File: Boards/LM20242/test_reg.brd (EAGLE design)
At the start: 160 x 100 mm, 12 parts, among them U1 TI_NATIONAL_SEMICONDUCTOR_LM2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

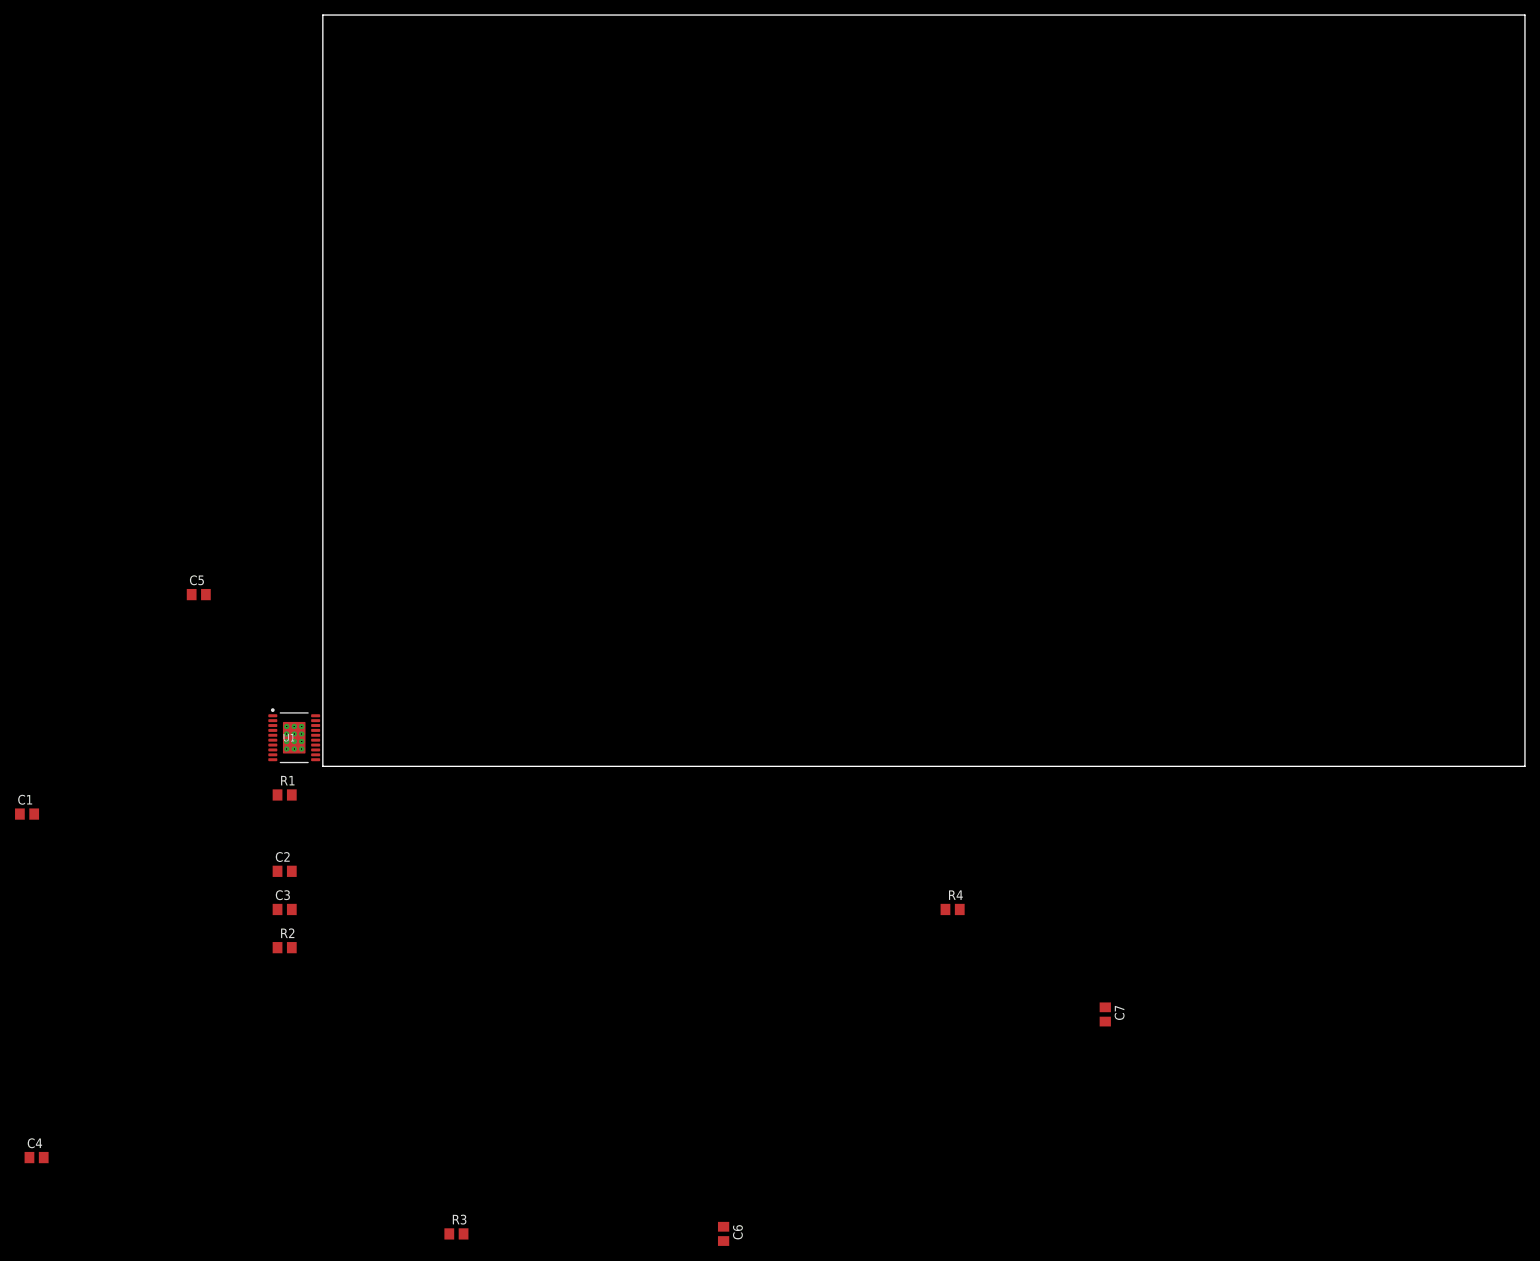
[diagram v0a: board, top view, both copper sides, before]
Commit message: routed board...?
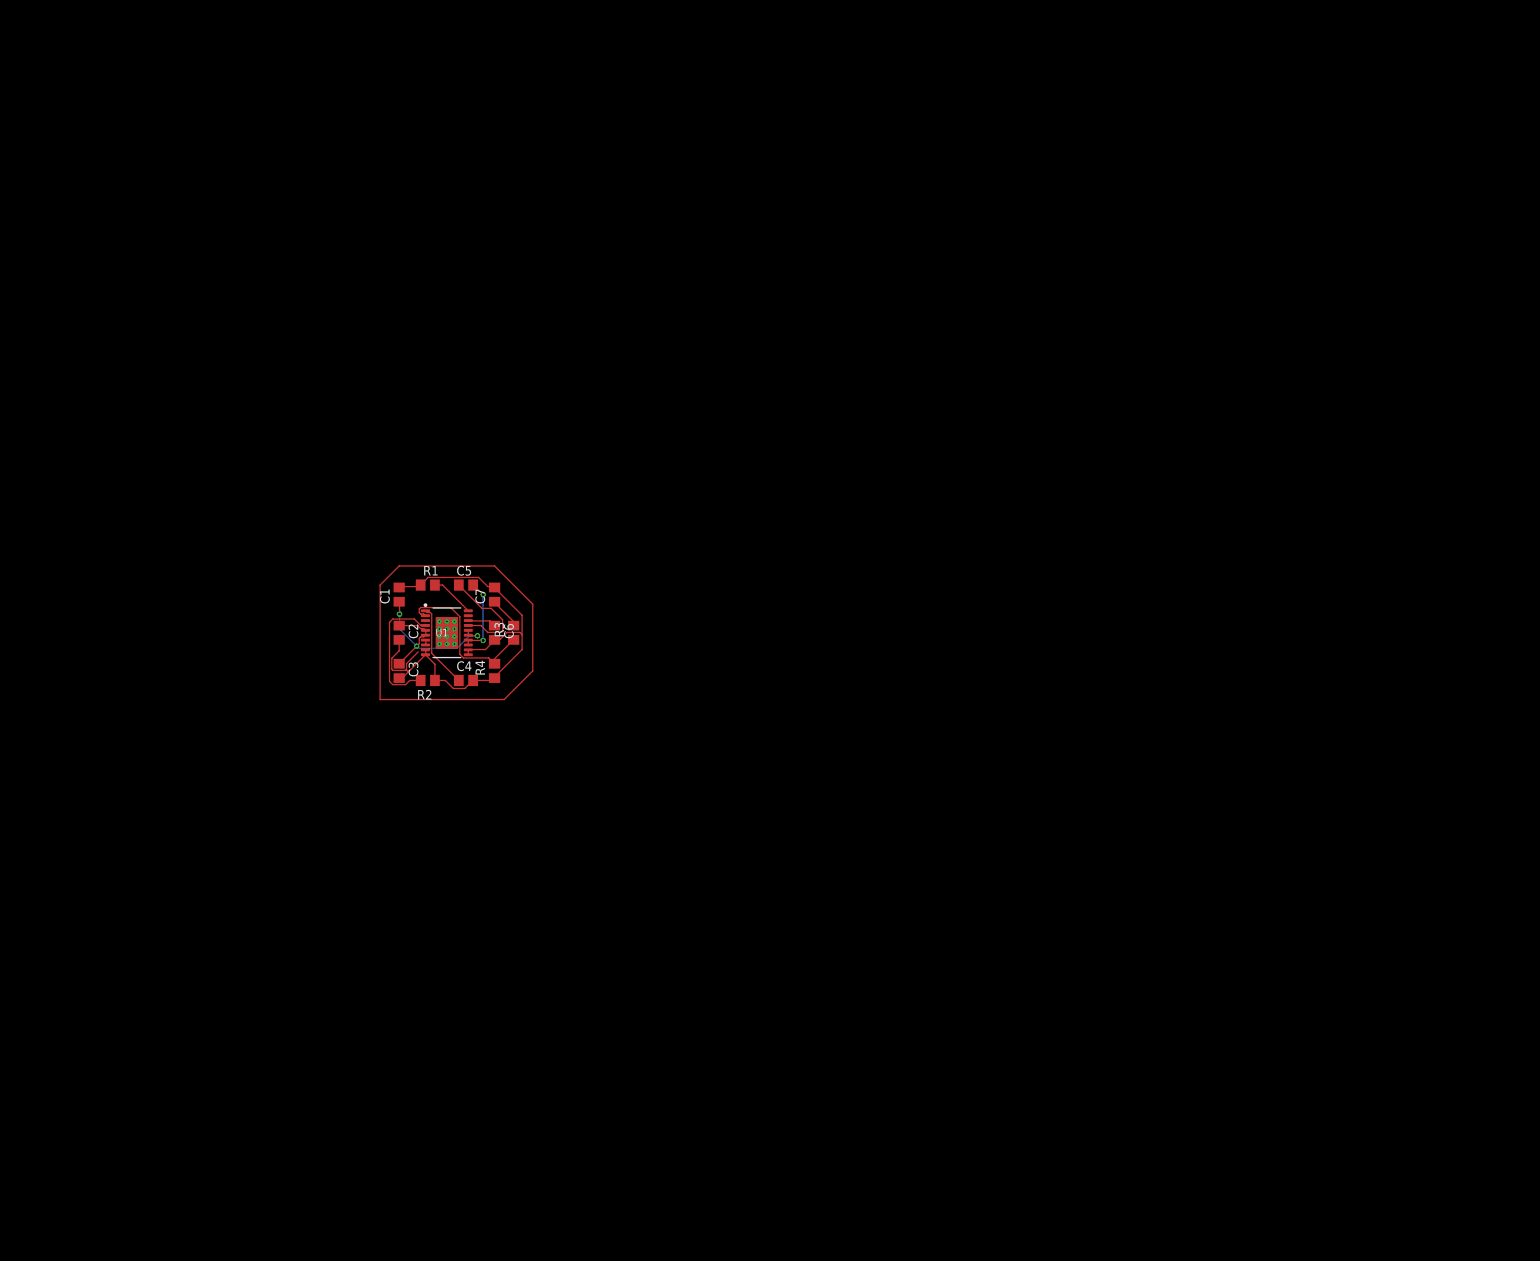
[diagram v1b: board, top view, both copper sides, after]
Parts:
- moved C7 98.6 mm to (22.9, 22.9), turned to 90 degrees
- moved C6 85.6 mm to (22.9, 17.8)
- moved C4 85.4 mm to (19.1, 11.4)
- moved R3 80.4 mm to (25.4, 17.8), turned to 90 degrees
- moved R4 68.7 mm to (22.9, 12.7), turned to 90 degrees
- moved C1 57.5 mm to (10.2, 22.9), turned to 90 degrees
- moved R2 40.3 mm to (14.0, 11.4), turned to 180 degrees
- moved C5 35.6 mm to (19.1, 24.1)
- moved C2 35.2 mm to (10.2, 17.8), turned to 270 degrees
- moved C3 35.2 mm to (10.2, 12.7), turned to 270 degrees
- moved R1 33.8 mm to (14.0, 24.1)
- moved U1 24.7 mm to (16.5, 17.8)
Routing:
- net N$7: track 0.00 -> 69.5 mm
- net GND: track 0.00 -> 66.2 mm
- net VCC: track 0.00 -> 27.6 mm, vias 0 -> 3
- net N$6: track 0.00 -> 22.1 mm
- net N$2: track 0.00 -> 17.7 mm
- net N$5: track 0.00 -> 14.3 mm
- net N$3: track 0.00 -> 11.4 mm
- net N$4: track 0.00 -> 11.3 mm, vias 0 -> 2
- net N$1: track 0.00 -> 5.86 mm
- net VOUT: track 0.00 -> 4.28 mm
- net N$9: track 0.00 -> 3.78 mm
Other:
- board outline removed
